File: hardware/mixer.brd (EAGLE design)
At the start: 100 x 100 mm, 261 parts, among them IC1 PGA2311, IC10 OPA2134P, IC11 OPA2134P, IC12 OPA2134P, IC13 OPA2134P, IC14 PGA2311, IC2 PGA2311, IC3 PGA2311, IC4 PGA2311, IC5 PGA2311, IC6 OPA2134P, IC7 OPA2134P, IC8 OPA2134P, IC9 OPA2134P, Q1 SI2305, T1 BC846, U1 V_REG_LDOSMD, X1 MOLEX_6HORIZONTAL, X3 display, X4 input, X5 2512-5, X6 2512-5, Y1 32768Hz CFPX-217 12.5pF

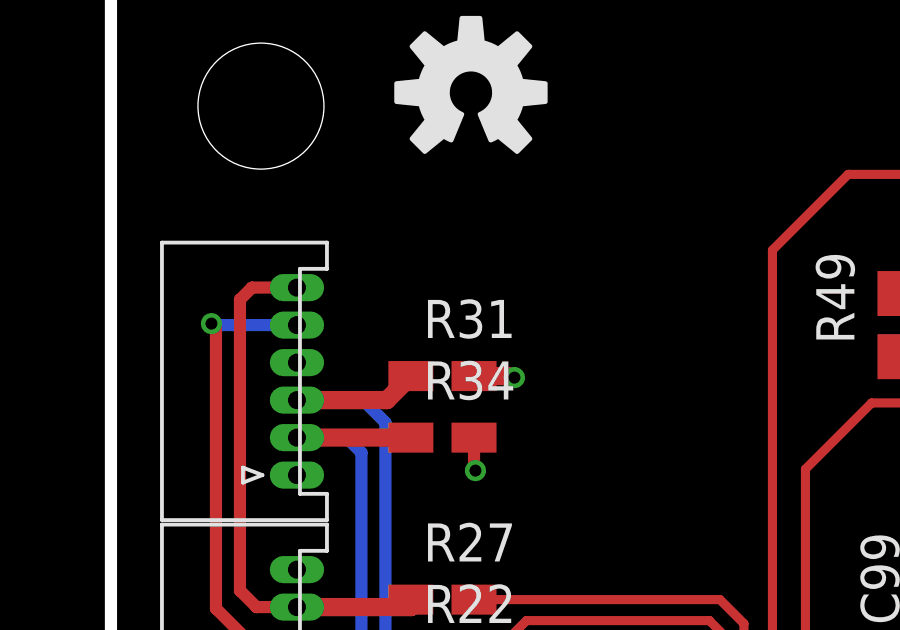
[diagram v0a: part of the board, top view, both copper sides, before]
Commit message: new power amp
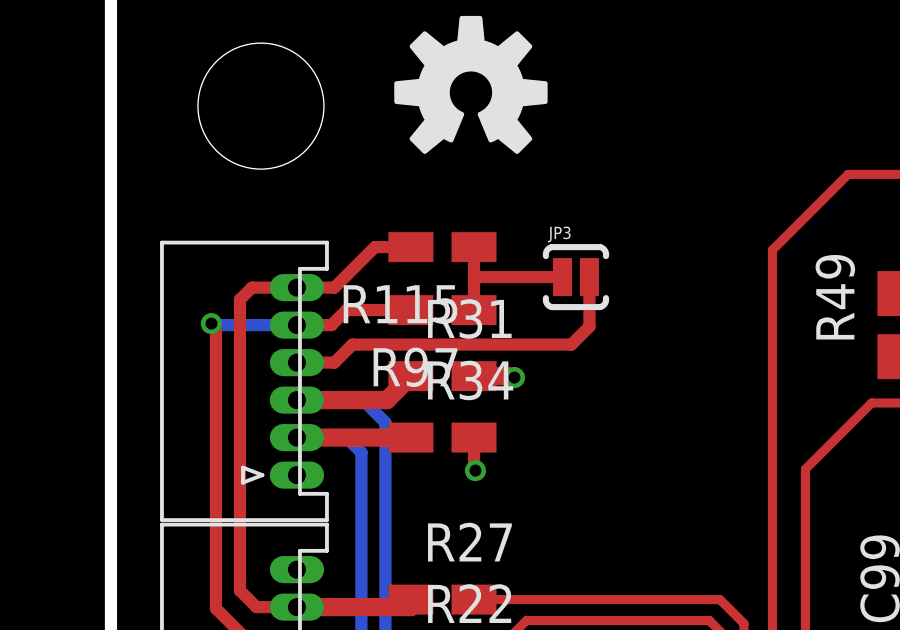
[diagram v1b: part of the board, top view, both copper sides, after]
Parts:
- added JP3: (no value), SparkFun-Passives:SJ_2S-NO
- added R115, R97: NA/4K7, rcl:R0805W
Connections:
- net N$14 renamed P4.5
- net N$21 renamed P4.4
- removed net RX: R22.1, X1.5, X3.2
- removed net TX: R27.1, X1.6, X3.3
- new net N$13: JP3.1, R115.1, R97.1
- new net RX/SDA: R22.1, R97.2, X1.5, X3.2
- new net TX/SCL: R115.2, R27.1, X1.6, X3.3
- net 3V3: now also JP3.2
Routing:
- net RX/SDA: track 0.00 -> 24.0 mm, vias 0 -> 1
- net TX/SCL: track 0.00 -> 22.3 mm
- net RX: track 20.0 -> 0.00 mm, vias 1 -> 0
- net TX: track 17.9 -> 0.00 mm
- net 3V3: track 150.9 -> 162.8 mm
- net N$13: track 0.00 -> 5.09 mm
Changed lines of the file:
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@@
 <element name="R79" library="rcl" package="R0805W" value="10K" x="49.17" y="13.34" rot="R180"/>
 <element name="R96" library="rcl" package="R0805W" value="10K" x="49.15" y="15.54" rot="R180"/>
+<element name="R97" library="rcl" package="R0805W" value="NA/4K7" x="11.05" y="88.2" rot="R180"/>
+<element name="R115" library="rcl" package="R0805W" value="NA/4K7" x="11.05" y="90.3" rot="R180"/>
+<element name="JP3" library="SparkFun-Passives" package="SJ_2S-NO" value="" x="15.5" y="89.3"/>
 </elements>
 <signals>
@@
 <wire x1="11.15" y1="61.55" x2="10.15" y2="61.55" width="0.3048" layer="1"/>
 </signal>
-<signal name="N$14">
+<signal name="P4.5">
 <contactref element="U$11" pad="34"/>
 <contactref element="R22" pad="2"/>
@@
 <wire x1="12.5" y1="76.5" x2="12.1025" y2="76.5" width="0.3048" layer="1"/>
 </signal>
-<signal name="N$21">
+<signal name="P4.4">
 <contactref element="U$11" pad="33"/>
 <contactref element="R27" pad="2"/>
@@
 <wire x1="20.6" y1="68.5" x2="18.55" y2="68.5" width="0.3048" layer="1"/>
 </signal>
-<signal name="RX">
+<signal name="RX/SDA">
 <contactref element="R22" pad="1"/>
 <contactref element="X1" pad="5"/>
@@
 <wire x1="6.2" y1="87.7" x2="3.4" y2="87.7" width="0.4064" layer="16"/>
 <wire x1="3.4" y1="87.7" x2="3.35" y2="87.75" width="0.4064" layer="16"/>
+<contactref element="R97" pad="2"/>
+<wire x1="9.9975" y1="88.2" x2="7.85" y2="88.2" width="0.4064" layer="1"/>
+<wire x1="7.85" y1="88.2" x2="7.35" y2="87.7" width="0.4064" layer="1"/>
+<wire x1="7.35" y1="87.7" x2="6.2" y2="87.7" width="0.4064" layer="1"/>
 </signal>
-<signal name="TX">
+<signal name="TX/SCL">
 <contactref element="R27" pad="1"/>
 <contactref element="X1" pad="6"/>
@@
 <wire x1="4.3" y1="88.55" x2="4.7" y2="88.95" width="0.4064" layer="1"/>
 <wire x1="4.7" y1="88.95" x2="6.2" y2="88.95" width="0.4064" layer="1"/>
+<contactref element="R115" pad="2"/>
+<wire x1="6.2" y1="88.95" x2="7.45" y2="88.95" width="0.4064" layer="1"/>
+<wire x1="7.45" y1="88.95" x2="8.8" y2="90.3" width="0.4064" layer="1"/>
+<wire x1="8.8" y1="90.3" x2="9.9975" y2="90.3" width="0.4064" layer="1"/>
 </signal>
 <signal name="N$30">
@@
 <wire x1="20.8" y1="63.5" x2="20.8" y2="65.6" width="0.4064" layer="1"/>
 <wire x1="20.8" y1="65.6" x2="20.75" y2="65.65" width="0.4064" layer="1"/>
+<wire x1="8.05" y1="87.05" x2="7.45" y2="86.45" width="0.4064" layer="1"/>
+<wire x1="7.45" y1="86.45" x2="6.2" y2="86.45" width="0.4064" layer="1"/>
+<contactref element="JP3" pad="2"/>
+<wire x1="8.05" y1="87.05" x2="15.35" y2="87.05" width="0.4064" layer="1"/>
+<wire x1="15.35" y1="87.05" x2="15.95" y2="87.65" width="0.4064" layer="1"/>
+<wire x1="15.95" y1="87.65" x2="15.95" y2="89.3" width="0.4064" layer="1"/>
 </signal>
 <signal name="CENTER">
@@
 <contactref element="U$11" pad="43"/>
 </signal>
+<signal name="N$13">
+<contactref element="R97" pad="1"/>
+<contactref element="R115" pad="1"/>
+<wire x1="12.1025" y1="90.3" x2="12.1025" y2="89.4" width="0.4064" layer="1"/>
+<contactref element="JP3" pad="1"/>
+<wire x1="12.1025" y1="89.4" x2="12.1025" y2="88.2" width="0.4064" layer="1"/>
+<wire x1="15.05" y1="89.3" x2="12.2025" y2="89.3" width="0.4064" layer="1"/>
+<wire x1="12.2025" y1="89.3" x2="12.1025" y2="89.4" width="0.4064" layer="1"/>
+</signal>
 </signals>
